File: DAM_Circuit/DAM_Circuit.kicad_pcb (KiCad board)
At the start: 2 copper layers, 200 x 100 mm, 98 parts, among them J1 Screw_Terminal_01x02, J2 Screw_Terminal_01x02, J3 Power Source (12V), Q1 IRLZ44N, Q2 IRLZ44N, SW1 SW_Push, SW2 SW_Push, U1 74LS147, U10 74LS48, U11 74LS125, U12 74LS20, U13 74LS21, U14 74LS85, U15 74LS85, U16 74LS32, U17 A1104xLH, U18 A1104xLH, U19 A1104xLH, U2 74LS175, U20 A1104xLH, U21 A1104xLH, U22 A1104xLH, U23 A1104xLH, U24 A1104xLH, U25 A1104xLH, U26 A1104xLH, U27 SM420561N, U28 SM420561N, U29 LM7805_TO220, U3 74LS157, U4 74LS85, U5 74LS04, U6 74LS32, U7 74LS04, U8 74LS85, U9 74LS157

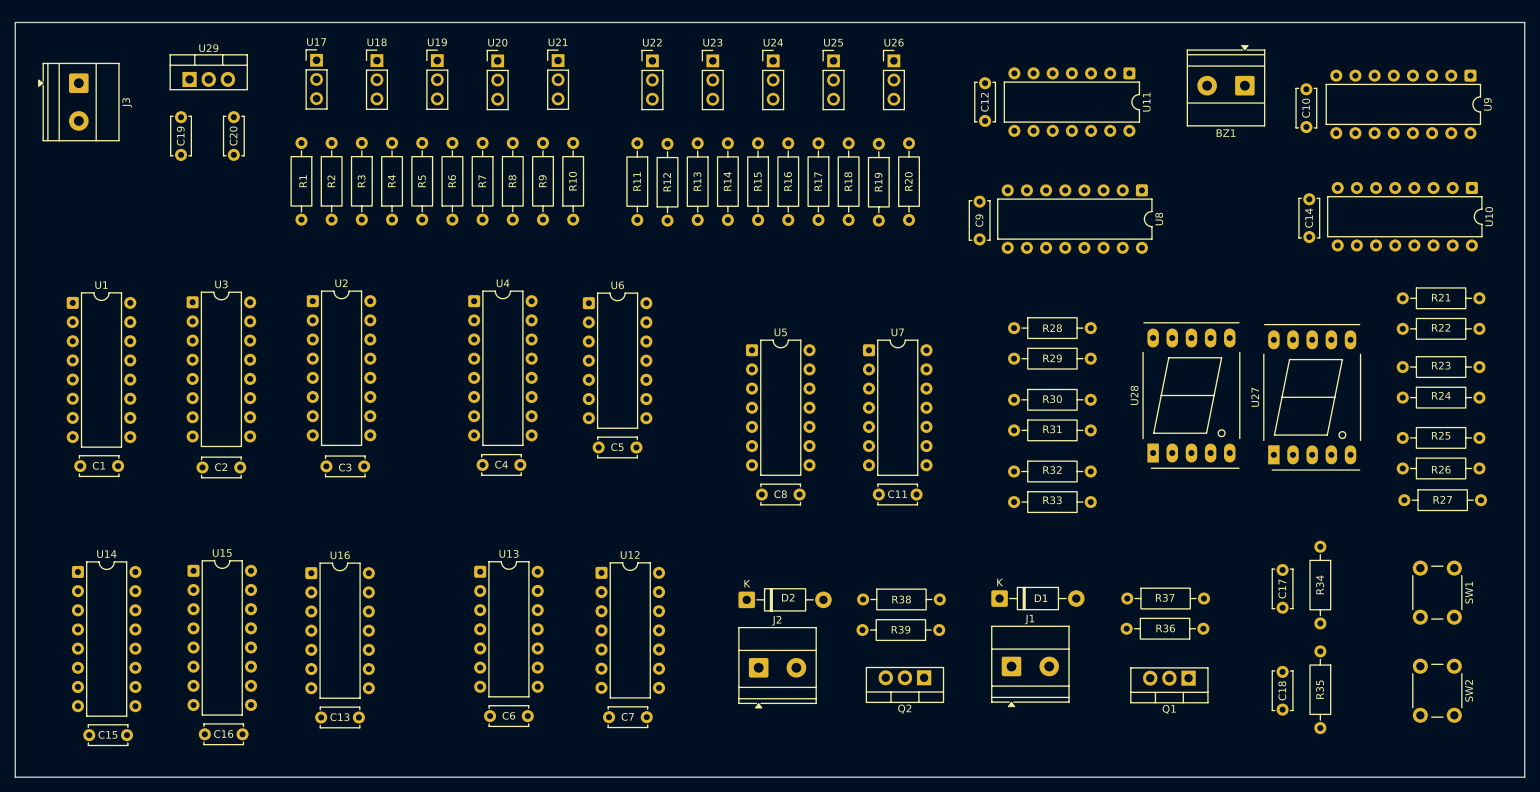
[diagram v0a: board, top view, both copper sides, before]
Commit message: 6.7.2026 already routed, need to compress more
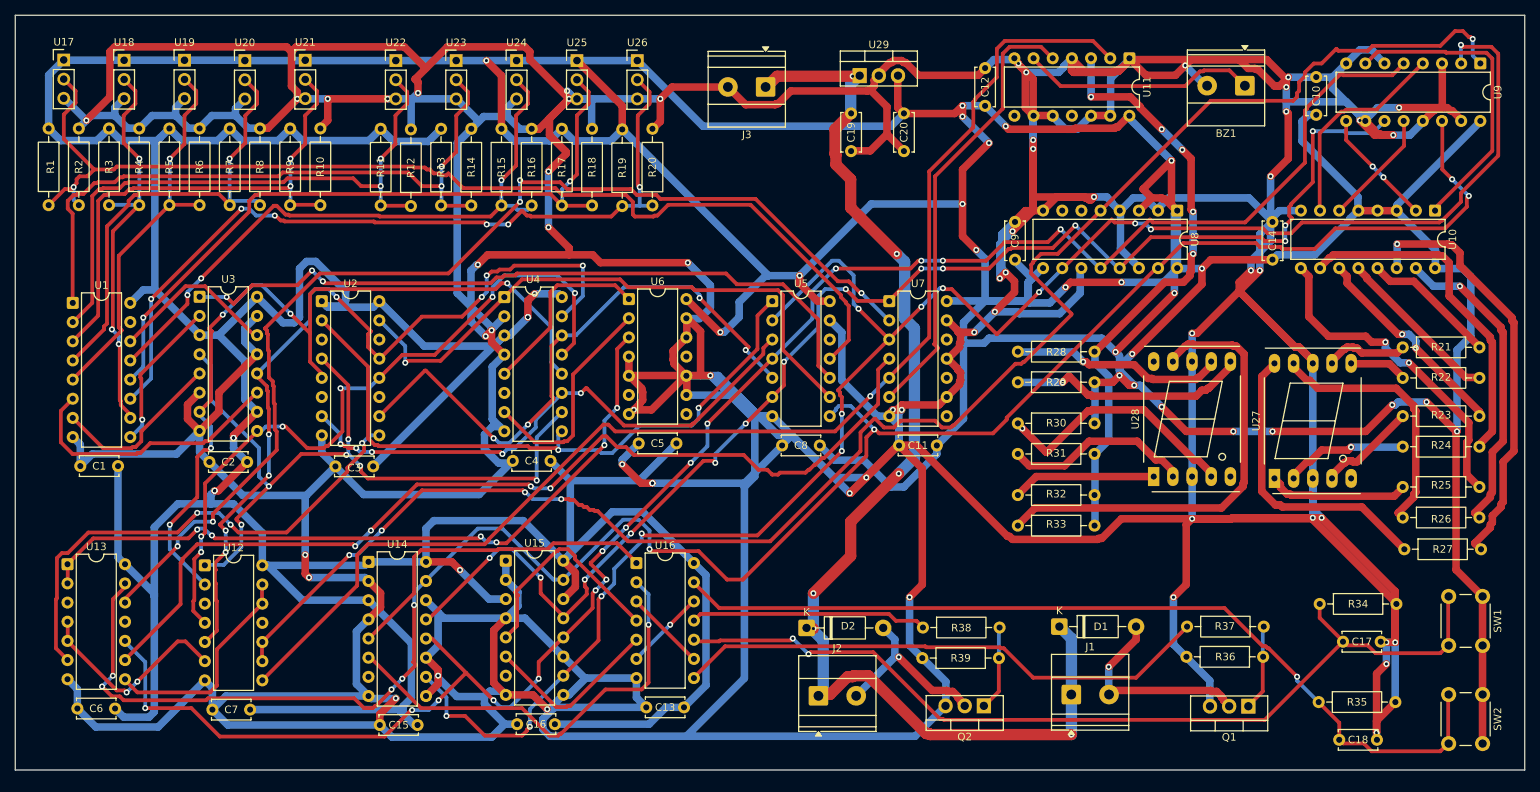
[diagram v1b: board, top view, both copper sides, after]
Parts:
- moved J3 91.0 mm to (200.5, 94.5), turned to 180 degrees
- moved U29 88.8 mm to (213.0, 93.0)
- moved C20 88.8 mm to (218.8, 103.0)
- moved C19 88.8 mm to (211.8, 103.0)
- moved C6 54.7 mm to (109.3, 176.9)
- moved U13 54.7 mm to (108.0, 157.7)
- moved C7 52.6 mm to (127.2, 177.0)
- moved U12 52.6 mm to (126.2, 157.9)
- moved C13 43.1 mm to (184.7, 176.7)
- moved U16 43.1 mm to (183.4, 157.6)
- moved C16 41.4 mm to (167.6, 178.9)
- moved U15 41.4 mm to (166.1, 157.3)
- moved C15 38.5 mm to (149.4, 179.0)
- moved U14 38.5 mm to (147.9, 157.4)
- moved R12 34.1 mm to (153.5, 110.3)
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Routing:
- net GND: track 0.00 -> 1758.0 mm, vias 0 -> 58
- net +5V: track 0.00 -> 1225.9 mm, vias 0 -> 32
- net D: track 0.00 -> 268.1 mm, vias 0 -> 9
- net B: track 0.00 -> 246.0 mm, vias 0 -> 15
- net A: track 0.00 -> 245.0 mm, vias 0 -> 13
- net Net-(U8-Oa>b): track 0.00 -> 222.6 mm, vias 0 -> 5
- net C: track 0.00 -> 183.7 mm, vias 0 -> 14
- net Net-(U11-Pad2): track 0.00 -> 169.1 mm, vias 0 -> 1
- net +12V: track 0.00 -> 161.1 mm, vias 0 -> 6
- net Net-(U13-Pad12): track 0.00 -> 147.0 mm, vias 0 -> 5
- net P10: track 0.00 -> 144.6 mm, vias 0 -> 1
- net Net-(U13-Pad9): track 0.00 -> 128.8 mm, vias 0 -> 4
- net Net-(C17-Pad1): track 0.00 -> 123.3 mm, vias 0 -> 2
- net Net-(C18-Pad1): track 0.00 -> 118.0 mm, vias 0 -> 1
- net Net-(U2-D1): track 0.00 -> 112.1 mm, vias 0 -> 5
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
